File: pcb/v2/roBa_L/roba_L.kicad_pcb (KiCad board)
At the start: 2 copper layers, 123.9 x 94.5 mm, 56 parts, among them J1 Conn_01x01-Connector_Generic, J2 Conn_01x01-Connector_Generic, J3 Conn_01x01-Connector_Generic, J4 Conn_01x01-Connector_Generic, J5 Conn_01x01-Connector_Generic, J6 Conn_01x01-Connector_Generic, J7 Conn_01x01-Connector_Generic, SW1 SW_PUSH, SW10 SW_PUSH, SW11 SW_PUSH, SW12 SW_PUSH, SW13 SW_PUSH, SW14 SW_PUSH, SW15 SW_PUSH, SW16 SW_PUSH, SW17 SW_PUSH, SW18 SW_PUSH, SW19 SW_PUSH, SW2 SW_PUSH, SW20 SW_PUSH, SW21 RotaryEncoder_Switch, SW22 SW_PUSH, SW23 SW_PUSH, SW24 SW_SPDT, SW3 SW_PUSH, SW4 SW_PUSH, SW5 SW_PUSH, SW6 SW_PUSH, SW7 SW_PUSH, SW8 SW_PUSH, SW9 SW_PUSH

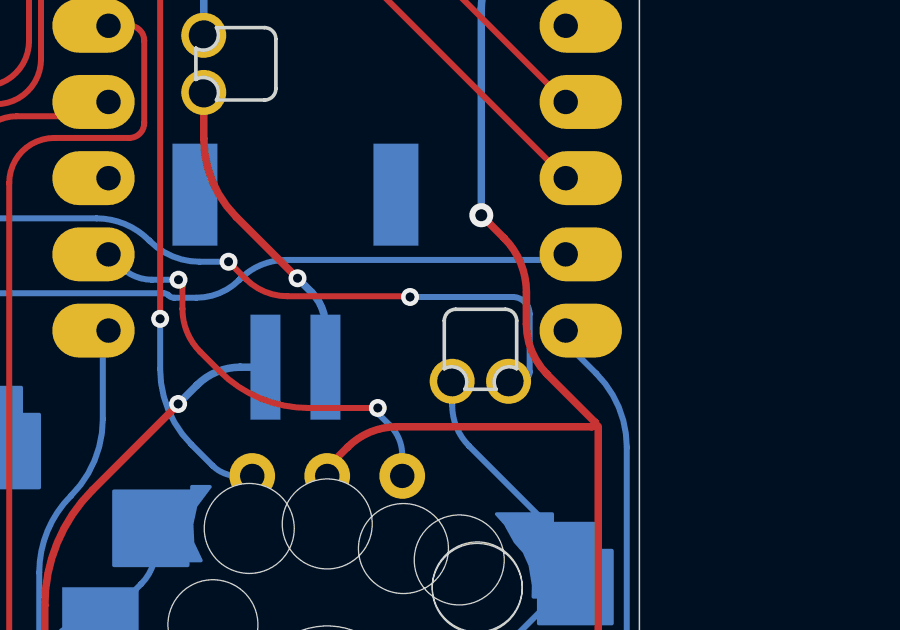
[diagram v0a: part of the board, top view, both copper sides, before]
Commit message: Redo pmw3610 sensor board
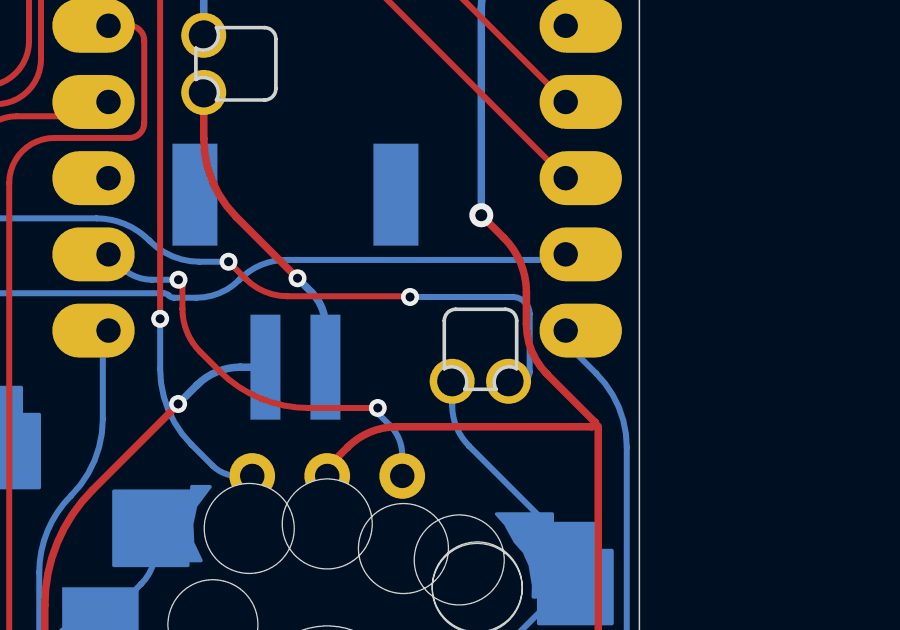
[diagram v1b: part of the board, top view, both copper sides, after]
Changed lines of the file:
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@@
 		(fp_arc
 			(start 3.572247 17.791753)
-			(mid 3.683838 17.522342)
+			(mid 3.683839 17.522346)
 			(end 3.953247 17.410753)
 			(stroke
